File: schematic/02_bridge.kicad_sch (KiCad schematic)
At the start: 54 parts, among them Q201 ISC011N06LM5, Q202 ISC011N06LM5, Q203 ISC011N06LM5, Q204 ISC011N06LM5, Q205 ISC011N06LM5, Q206 ISC011N06LM5, U202 INA241A2DR, U203 INA241A2DR, U204 INA241A2DR

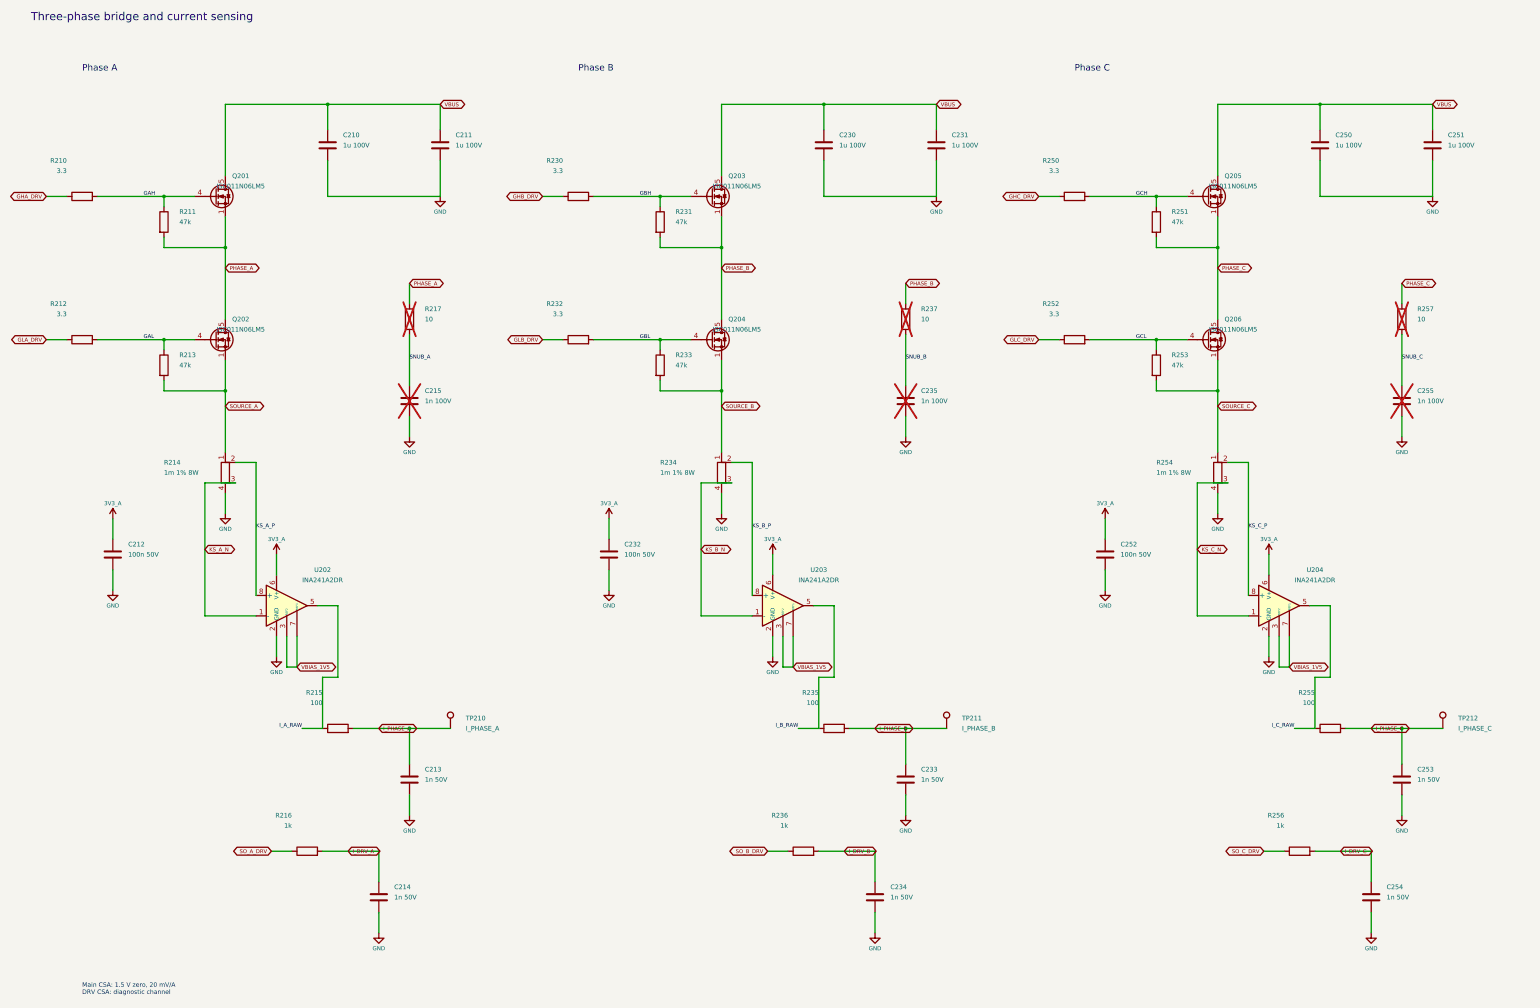
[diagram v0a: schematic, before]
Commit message: devlog 03
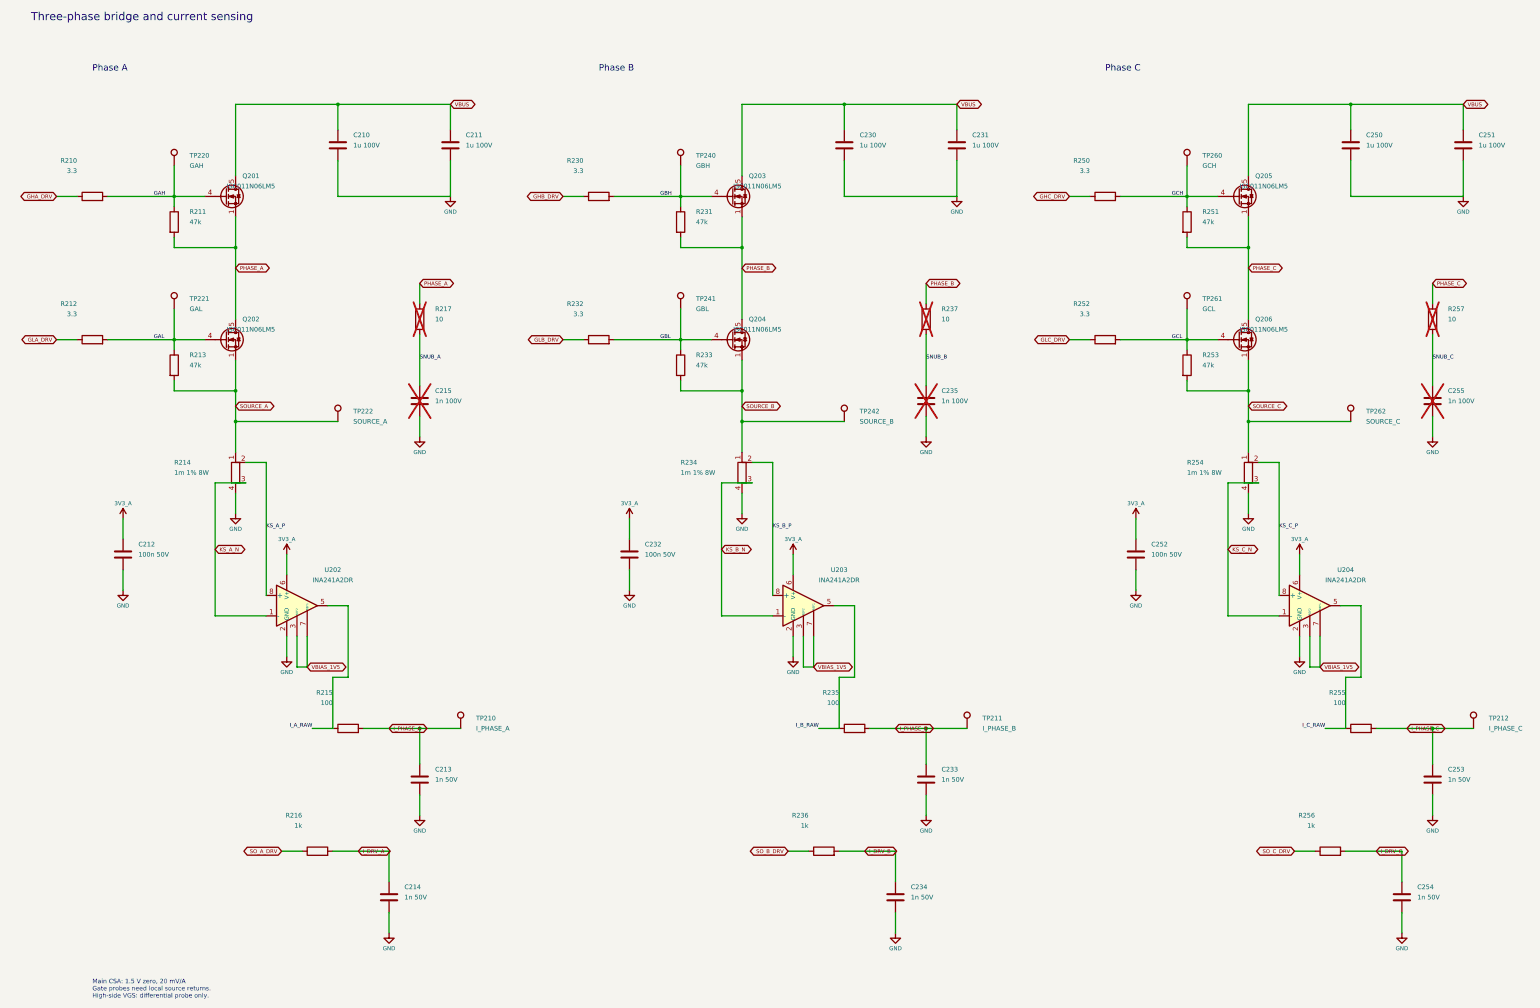
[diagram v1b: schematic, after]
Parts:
- added TP220: GAH, TestPoint:TestPoint_Pad_D1.5mm, symbol Connector:TestPoint
- added TP221: GAL, TestPoint:TestPoint_Pad_D1.5mm, symbol Connector:TestPoint
- added TP222: SOURCE_A, TestPoint:TestPoint_Pad_D1.5mm, symbol Connector:TestPoint
- added TP240: GBH, TestPoint:TestPoint_Pad_D1.5mm, symbol Connector:TestPoint
- added TP241: GBL, TestPoint:TestPoint_Pad_D1.5mm, symbol Connector:TestPoint
- added TP242: SOURCE_B, TestPoint:TestPoint_Pad_D1.5mm, symbol Connector:TestPoint
- added TP260: GCH, TestPoint:TestPoint_Pad_D1.5mm, symbol Connector:TestPoint
- added TP261: GCL, TestPoint:TestPoint_Pad_D1.5mm, symbol Connector:TestPoint
- added TP262: SOURCE_C, TestPoint:TestPoint_Pad_D1.5mm, symbol Connector:TestPoint
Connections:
- net GAH: now also TP220.1
- net GAL: now also TP221.1
- net GBH: now also TP240.1
- net GBL: now also TP241.1
- net GCH: now also TP260.1
- net GCL: now also TP261.1
- net SOURCE_A: now also TP222.1
- net SOURCE_B: now also TP242.1
- net SOURCE_C: now also TP262.1
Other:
- note added: "Main CSA: 1.5 V zero, 20 mV/A Gate probes need local source returns. High-side VGS: differential probe only."
- note removed: "Main CSA: 1.5 V zero, 20 mV/A DRV CSA: diagnostic channel"
- moved on the sheet: C210, C211, C212, C213, C214, C215, C230, C231, C232, C233, C234, C235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
